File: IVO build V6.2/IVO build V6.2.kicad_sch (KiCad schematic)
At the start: 15 parts, among them Q2 C2M0080120D, U1 L7805, U2 1EDI60I12AF, U3 MGJ1D121505MPC-R7

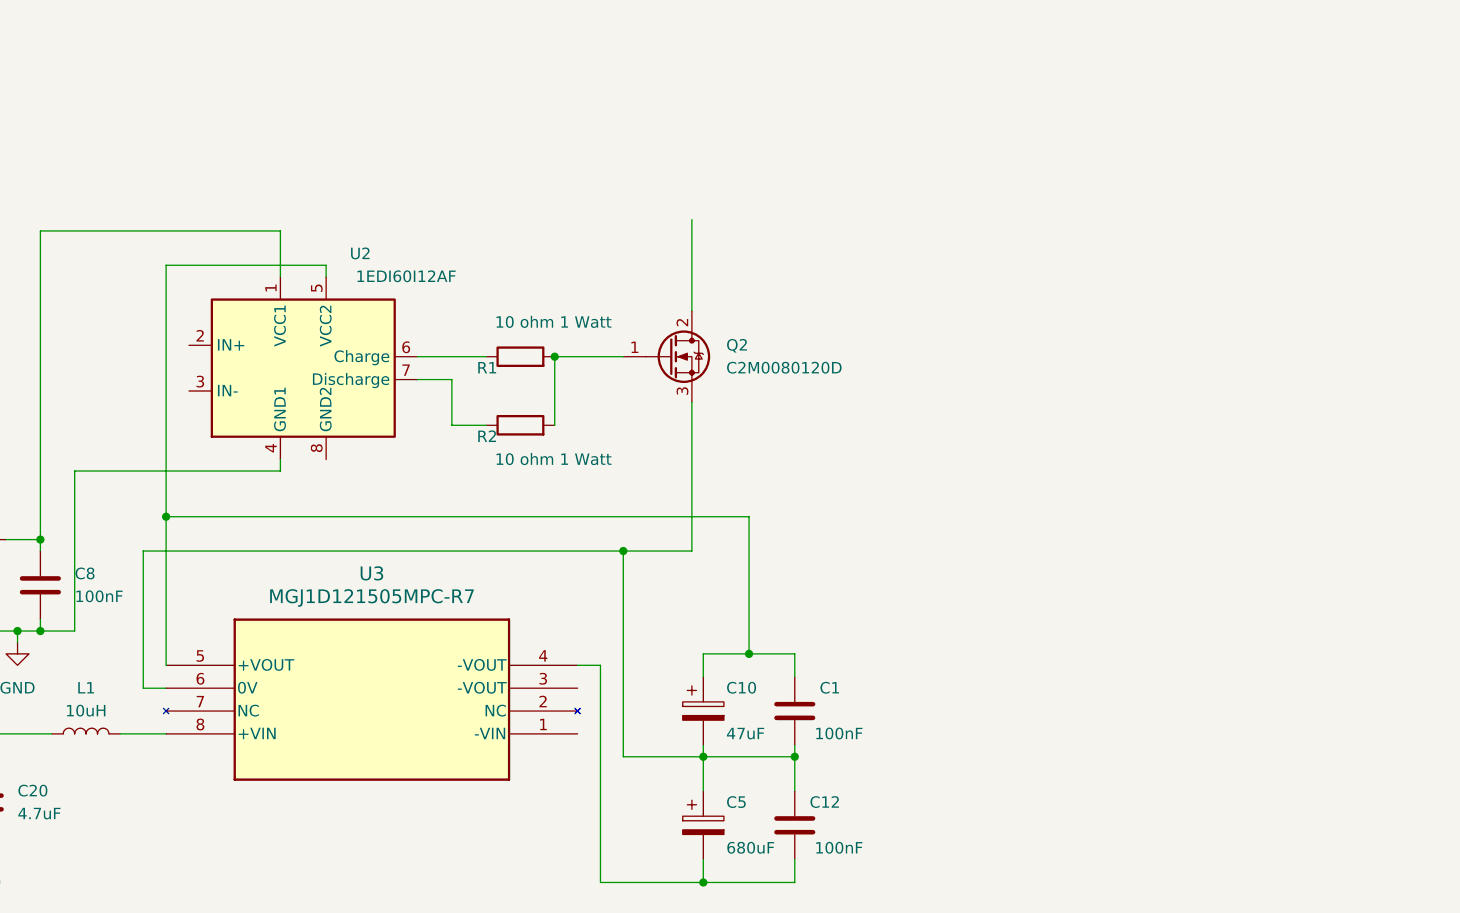
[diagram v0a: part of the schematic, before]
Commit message: updated schematic and added picture
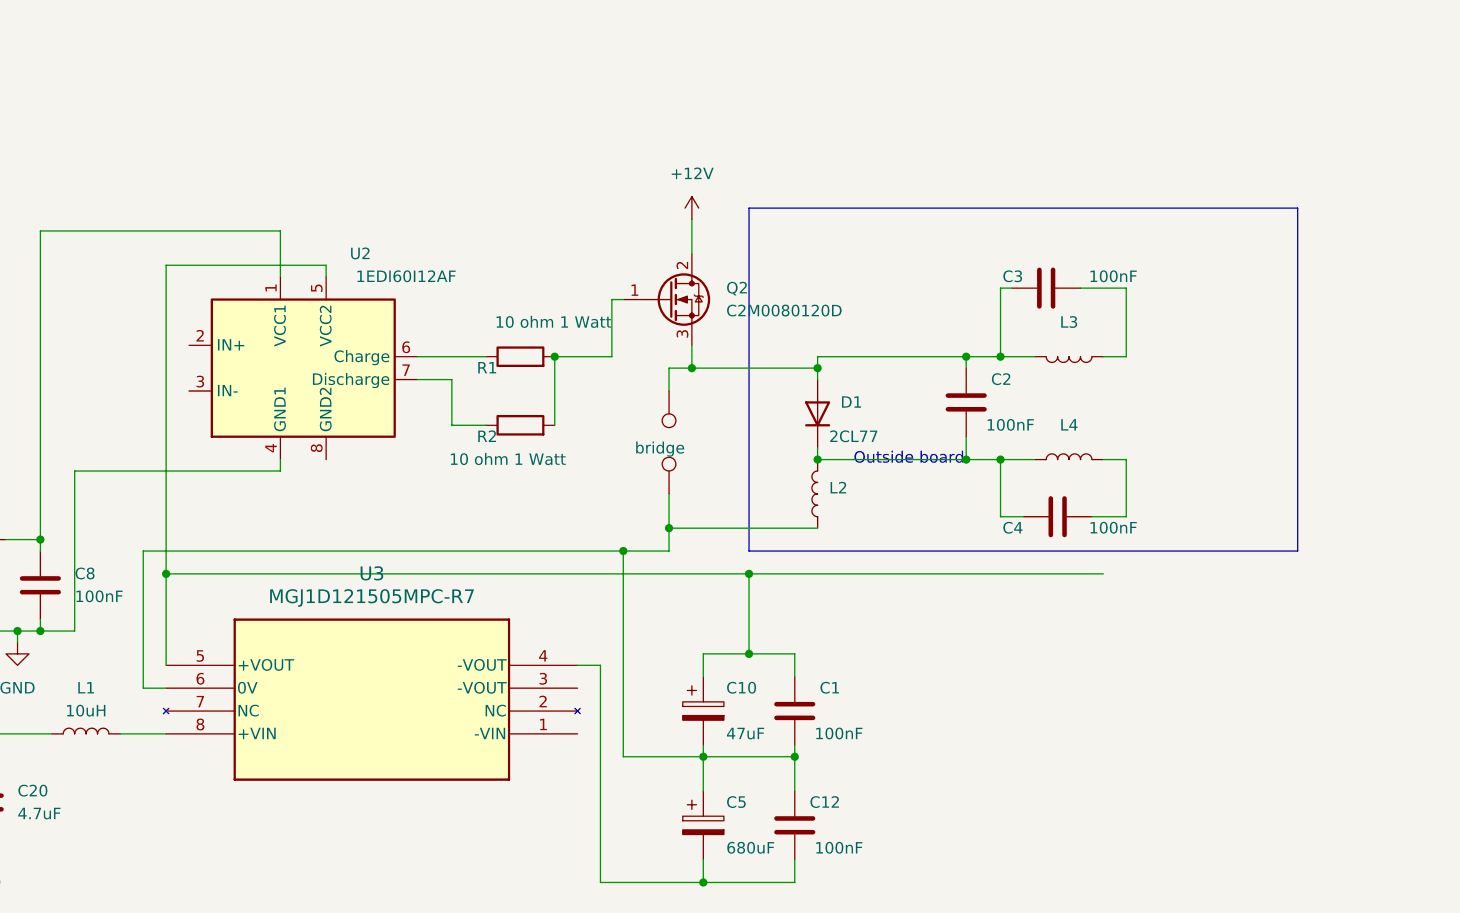
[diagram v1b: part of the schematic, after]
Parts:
- added C2, C3, C4: 100nF, symbol Device:C
- added D1: 2CL77, symbol Device:D
- added L2, L3, L4: ~, symbol Device:L
- added TP1: TestPoint, symbol Connector:TestPoint
- added TP2: bridge, symbol Connector:TestPoint
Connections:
- net +12V: now also Q2.2 (D)
- net at C1.2, C10.2, C12.1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: now also L2.1, TP2.1; no longer Q2.3 (S)
- new net: C2.1, C3.1, D1.2 (A), L3.2, Q2.3 (S), TP1.1
- new net: C3.2, L3.1
- new net: C2.2, C4.1, D1.1 (K), L2.2, L4.1
- new net: C4.2, L4.2
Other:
- note added: "Outside board"
- moved on the sheet: Q2
